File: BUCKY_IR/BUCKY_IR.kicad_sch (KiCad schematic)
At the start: 35 parts, among them J1 SERIAL_CONN, J2 CAN_CONN_UP, J3 CAN_CONN_DOWN, J4 PHOTODIODE, J5 LED, U1 TSSP96038TR, U10 TSSP96038TR, U11 TSSP96038TR, U12 TSSP96038TR, U13 TSSP96038TR, U14 TSSP96038TR, U15 TSSP96038TR, U16 TSSP96038TR, U17 SN65HVD230, U18 ESP32-WROOM-32U, U19 AMS1117-5.0, U2 TSSP96038TR, U3 TSSP96038TR, U4 TSSP96038TR, U5 TSSP96038TR, U6 TSSP96038TR, U7 TSSP96038TR, U8 TSSP96038TR, U9 TSSP96038TR

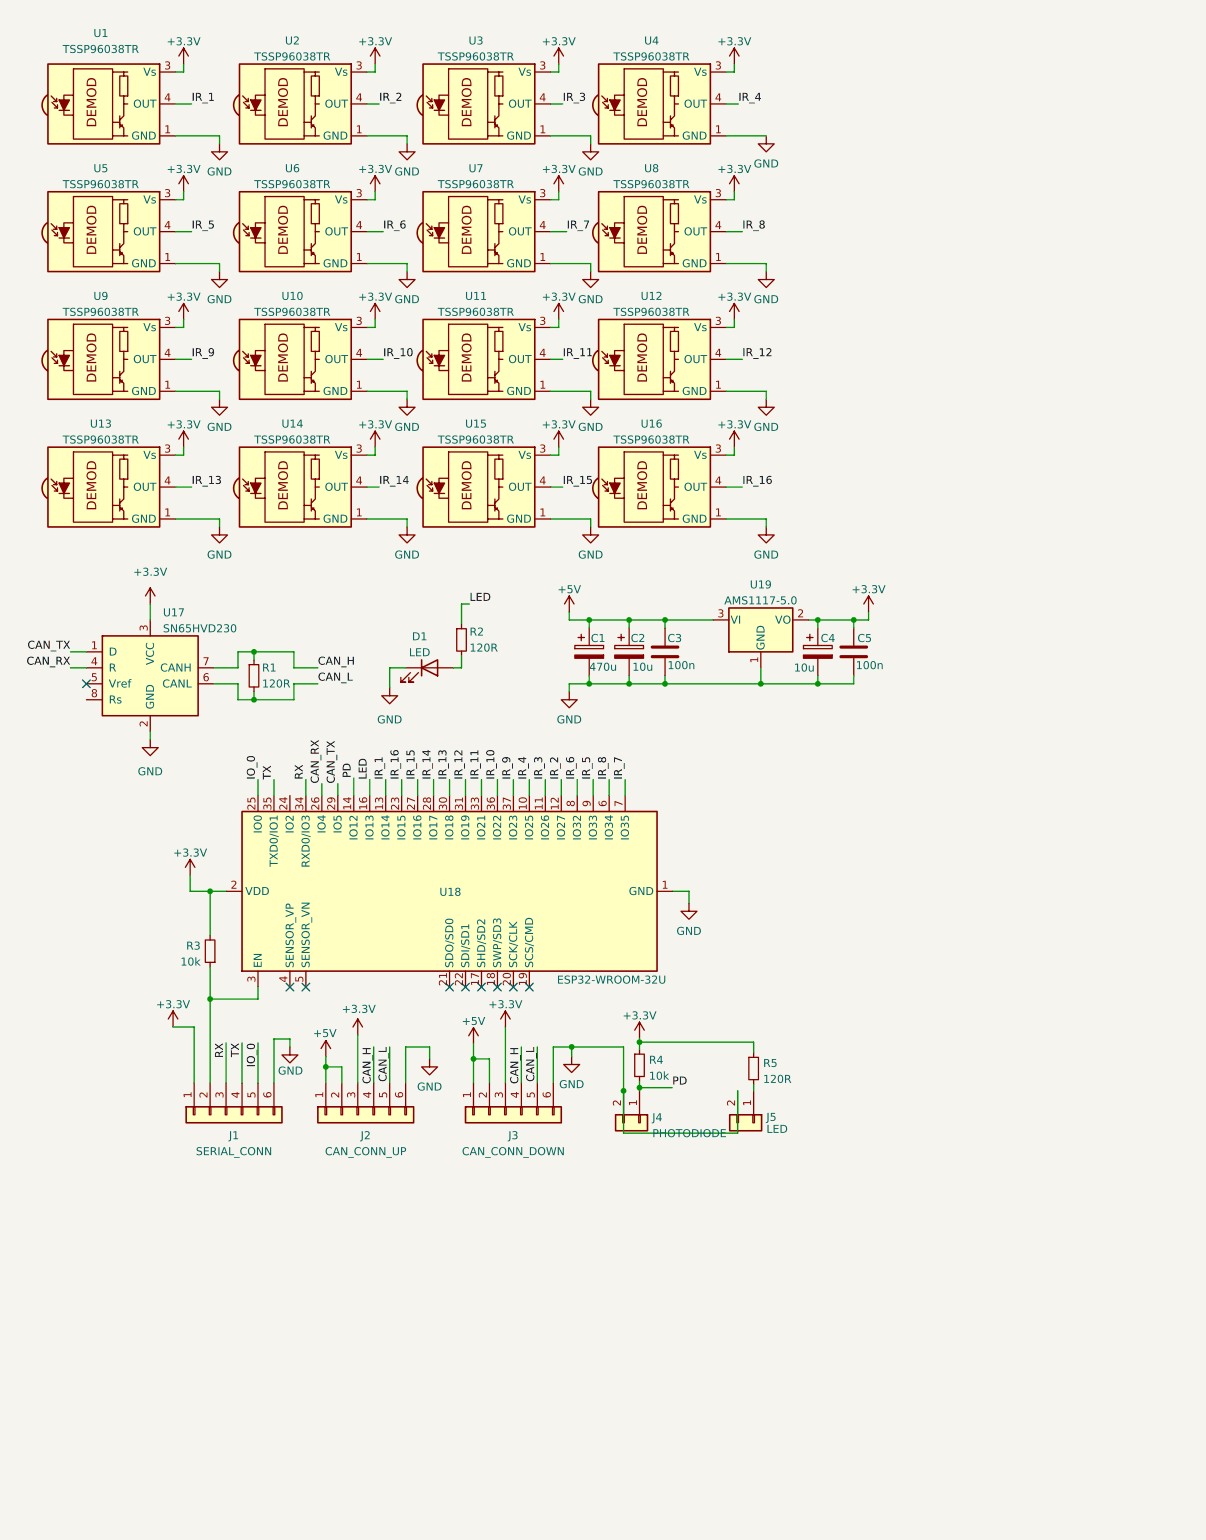
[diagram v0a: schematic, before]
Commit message: chore: start on schematics
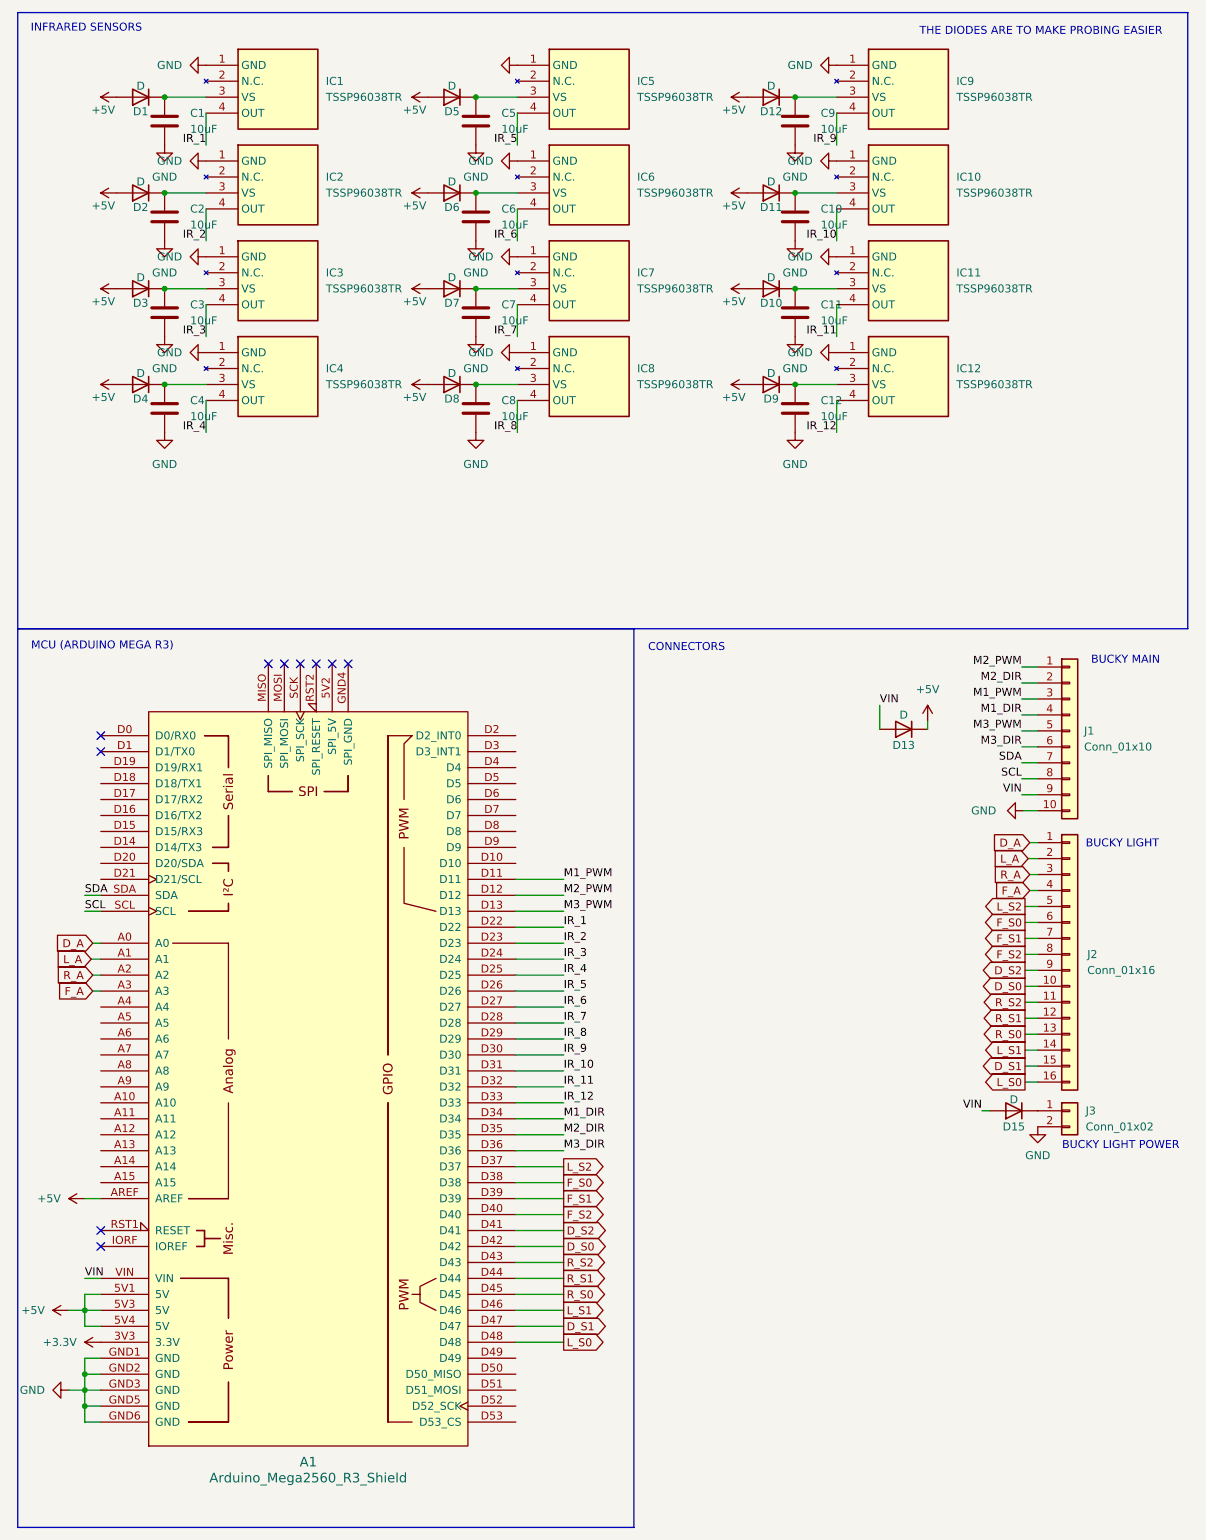
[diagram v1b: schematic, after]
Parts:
- removed C1: 470u, Capacitor_SMD:CP_Elec_6.3x7.7, symbol Device:C_Polarized
- removed C2, C4: 10u, Capacitor_SMD:CP_Elec_6.3x7.7, symbol Device:C_Polarized
- removed D1: LED, LED_SMD:LED_0805_2012Metric_Pad1.15x1.40mm_HandSolder, symbol Device:LED
- removed J1: SERIAL_CONN, Connector_JST:JST_PH_S6B-PH-SM4-TB_1x06-1MP_P2.00mm_Horizontal, symbol Connector_Generic:Conn_01x06
- removed J2: CAN_CONN_UP, Connector_JST:JST_PH_S6B-PH-SM4-TB_1x06-1MP_P2.00mm_Horizontal, symbol Connector_Generic:Conn_01x06
- removed J3: CAN_CONN_DOWN, Connector_JST:JST_PH_S6B-PH-SM4-TB_1x06-1MP_P2.00mm_Horizontal, symbol Connector_Generic:Conn_01x06
- removed J4: PHOTODIODE, Connector_PinHeader_2.54mm:PinHeader_1x02_P2.54mm_Horizontal, symbol Connector_Generic:Conn_01x02
- removed J5: LED, Connector_PinHeader_2.54mm:PinHeader_1x02_P2.54mm_Horizontal, symbol Connector_Generic:Conn_01x02
- removed R1, R2, R5: 120R, Resistor_SMD:R_0805_2012Metric_Pad1.20x1.40mm_HandSolder, symbol Device:R_Small
- removed R3, R4: 10k, Resistor_SMD:R_0805_2012Metric_Pad1.20x1.40mm_HandSolder, symbol Device:R_Small
- removed U1, U10, U11, U12, U13, U14, U15, U16, U2, U3, U4, U5, U6, U7, U8, U9: TSSP96038TR, BUCKY_IR:TSSP96038, symbol BUCKY_IR:TSSP96038TR
- removed U17: SN65HVD230, Package_SO:SOIC-8_3.9x4.9mm_P1.27mm, symbol Interface_CAN_LIN:SN65HVD230
- removed U18: ESP32-WROOM-32U, RF_Module:ESP32-WROOM-32U, symbol RF_Module:ESP32-WROOM-32U
- removed U19: AMS1117-5.0, Package_TO_SOT_SMD:SOT-223-3_TabPin2, symbol Regulator_Linear:AMS1117-5.0
- added A1: Arduino_Mega2560_R3_Shield, PCM_arduino-library:Arduino_Mega2560_R3_Shield, symbol PCM_arduino-library:Arduino_Mega2560_R3_Shield
- added C1, C10, C11, C12, C2, C4, C6, C7, C8, C9: 10uF, symbol Device:C
- added D1, D10, D11, D12, D13, D15, D2, D3, D4, D5, D6, D7, D8, D9: D, symbol Device:D
- added IC1, IC10, IC11, IC12, IC2, IC3, IC4, IC5, IC6, IC7, IC8, IC9: TSSP96038TR, TSSP96038TR, symbol BUCKY_IR:TSSP96038TR
- added J1: Conn_01x10, BUCKY_MAIN:CONN10_S10B-PH_JST, symbol Connector_Generic:Conn_01x10
- added J2: Conn_01x16, symbol Connector_Generic:Conn_01x16
- added J3: Conn_01x02, symbol Connector_Generic:Conn_01x02
- C3, C5: value 100n -> 10uF; footprint Capacitor_SMD:C_0805_2012Metric_Pad1.18x1.45mm_HandSolder -> (none)
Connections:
- net +3V3 is gone; now on net GND: C5.1
- net +5V: now also A1.5V1 (5V), A1.5V3 (5V), A1.5V4 (5V), A1.AREF, D1.2 (A), D10.2 (A), D11.2 (A), D12.2 (A), D13.1 (K), D2.2 (A), D3.2 (A), D4.2 (A), D5.2 (A), D6.2 (A), D7.2 (A), D8.2 (A), D9.2 (A); no longer C3.1
- net GND: now also C3.1, A1.GND1 (GND), A1.GND2 (GND), A1.GND3 (GND), A1.GND5 (GND), A1.GND6 (GND), C1.1, C10.1, C11.1, C12.1, C2.1, C4.1, C6.1, C7.1, C8.1, C9.1, IC1.1 (GND), IC10.1 (GND), IC11.1 (GND), IC12.1 (GND), IC2.1 (GND), IC3.1 (GND), IC4.1 (GND), IC5.1 (GND), IC6.1 (GND), IC7.1 (GND), IC8.1 (GND), IC9.1 (GND), J1.10 (Pin_10), J3.2 (Pin_2); no longer C3.2, C5.2
- net IR_1: now also A1.D22, IC1.4 (OUT)
- net IR_10: now also A1.D31, IC10.4 (OUT)
- net IR_11: now also A1.D32, IC11.4 (OUT)
- net IR_12: now also A1.D33, IC12.4 (OUT)
- net IR_2: now also A1.D23, IC2.4 (OUT)
- net IR_3: now also A1.D24, IC3.4 (OUT)
- net IR_4: now also A1.D25, IC4.4 (OUT)
- net IR_5: now also A1.D26, IC5.4 (OUT)
- net IR_6: now also A1.D27, IC6.4 (OUT)
- net IR_7: now also A1.D28, IC7.4 (OUT)
- net IR_8: now also A1.D29, IC8.4 (OUT)
- net IR_9: now also A1.D30, IC9.4 (OUT)
- new net: D15.1 (K), J3.1 (Pin_1)
- new net: C3.2, D3.1 (K), IC3.3 (VS)
- new net: C8.2, D8.1 (K), IC8.3 (VS)
- new net: C4.2, D4.1 (K), IC4.3 (VS)
- new net: C10.2, D11.1 (K), IC10.3 (VS)
- new net: C2.2, D2.1 (K), IC2.3 (VS)
- new net: C11.2, D10.1 (K), IC11.3 (VS)
- new net: C6.2, D6.1 (K), IC6.3 (VS)
- new net: C9.2, D12.1 (K), IC9.3 (VS)
- new net: C5.2, D5.1 (K), IC5.3 (VS)
- new net: C7.2, D7.1 (K), IC7.3 (VS)
- new net: C1.2, D1.1 (K), IC1.3 (VS)
- new net: C12.2, D9.1 (K), IC12.3 (VS)
- new net +3.3V: A1.3V3 (3.3V)
- new net D_A: A1.A0, J2.1 (Pin_1)
- new net D_S0: A1.D42, J2.10 (Pin_10)
- new net D_S1: A1.D47, J2.15 (Pin_15)
- new net D_S2: A1.D41, J2.9 (Pin_9)
- new net F_A: A1.A3, J2.4 (Pin_4)
- new net F_S0: A1.D38, J2.6 (Pin_6)
- new net F_S1: A1.D39, J2.7 (Pin_7)
- new net F_S2: A1.D40, J2.8 (Pin_8)
- new net L_A: A1.A1, J2.2 (Pin_2)
- new net L_S0: A1.D48, J2.16 (Pin_16)
- new net L_S1: A1.D46, J2.14 (Pin_14)
- new net L_S2: A1.D37, J2.5 (Pin_5)
- new net M1_DIR: A1.D34, J1.4 (Pin_4)
- new net M1_PWM: A1.D11, J1.3 (Pin_3)
- new net M2_DIR: A1.D35, J1.2 (Pin_2)
- new net M2_PWM: A1.D12, J1.1 (Pin_1)
- new net M3_DIR: A1.D36, J1.6 (Pin_6)
- new net M3_PWM: A1.D13, J1.5 (Pin_5)
- new net R_A: A1.A2, J2.3 (Pin_3)
- new net R_S0: A1.D45, J2.13 (Pin_13)
- new net R_S1: A1.D44, J2.12 (Pin_12)
- new net R_S2: A1.D43, J2.11 (Pin_11)
- new net SCL: A1.SCL, J1.8 (Pin_8)
- new net SDA: A1.SDA, J1.7 (Pin_7)
- new net VIN: A1.VIN, D13.2 (A), D15.2 (A), J1.9 (Pin_9)
- no-connect marks 9 -> 10
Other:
- note added: "BUCKY LIGHT"
- note added: "BUCKY LIGHT POWER"
- note added: "BUCKY MAIN"
- note added: "CONNECTORS"
- note added: "INFRARED SENSORS"
- note added: "MCU (ARDUINO MEGA R3)"
- note added: "THE DIODES ARE TO MAKE PROBING EASIER"
- company: (none) -> koen1711
- title: (none) -> BUCKY IR
